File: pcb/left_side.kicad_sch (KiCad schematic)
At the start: 148 parts, among them J1 USB_C_Receptacle_USB2.0_14P, SW1 SW_Push, SW10 SW_Push, SW11 SW_Push, SW12 SW_Push, SW13 SW_Push, SW14 SW_Push, SW15 SW_Push, SW16 SW_Push, SW17 SW_Push, SW18 SW_Push, SW19 SW_Push, SW2 SW_Push, SW20 SW_Push, SW21 SW_Push, SW22 SW_Push, SW23 SW_Push, SW24 SW_Push, SW25 SW_Push, SW26 SW_Push, SW27 SW_Push, SW28 SW_Push, SW29 SW_Push, SW3 SW_Push, SW30 SW_Push, SW31 SW_Push, SW32 SW_Push, SW33 SW_Push, SW34 SW_Push, SW35 SW_Push, SW36 SW_Push, SW37 SW_Push, SW38 SW_Push, SW39 SW_Push, SW4 SW_Push, SW40 SW_Push, SW41 SW_Push, SW42 SW_Push, SW43 SW_Push, SW44 SW_Push, SW45 SW_Push, SW46 SW_Push, SW47 SW_Push, SW48 SW_Push, SW5 SW_Push, SW6 SW_Push, SW7 SW_Push, SW8 SW_Push, SW9 SW_Push

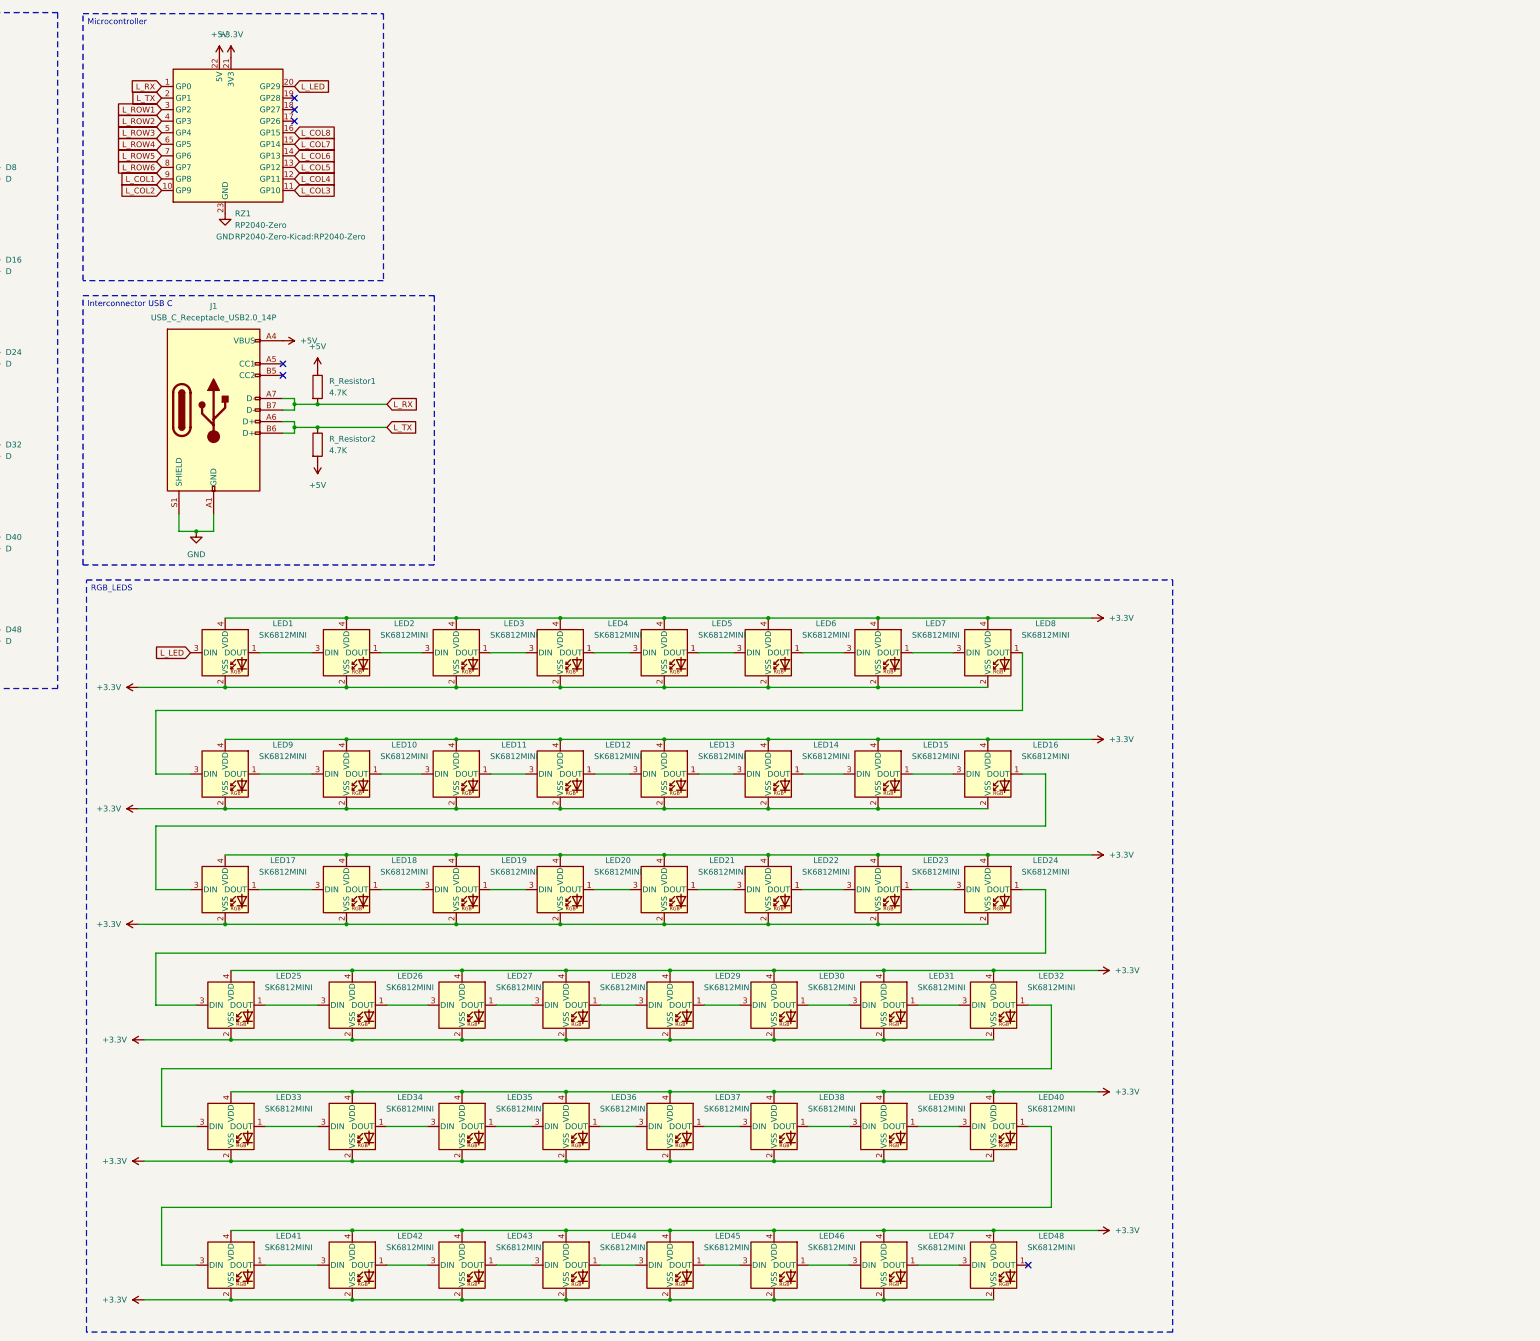
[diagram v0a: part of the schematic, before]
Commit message: update
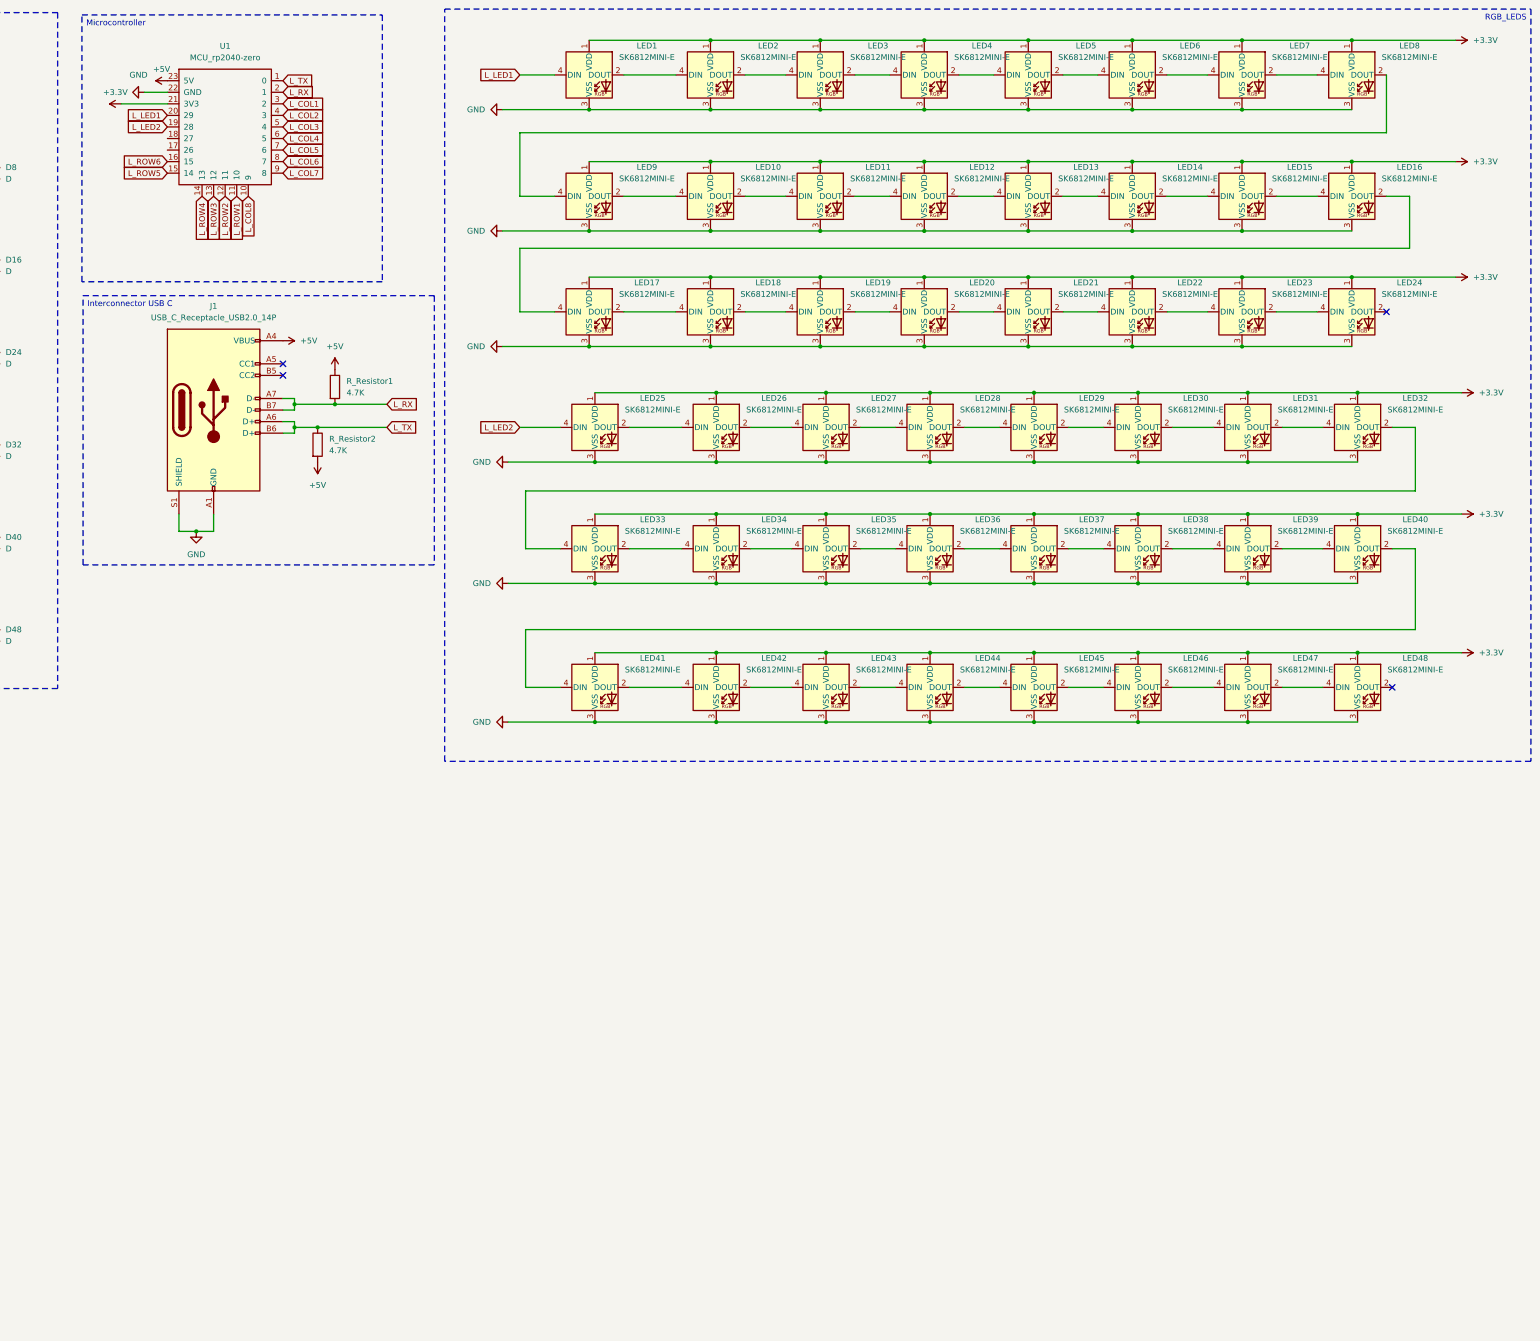
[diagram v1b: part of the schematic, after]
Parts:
- removed LED1, LED10, LED11, LED12, LED13, LED14, LED15, LED16, LED17, LED18, LED19, LED2, LED20, LED21, LED22, LED23, LED24, LED25, LED26, LED27, LED28, LED29, LED3, LED30, LED31, LED32, LED33, LED34, LED35, LED36, LED37, LED38, LED39, LED4, LED40, LED41, LED42, LED43, LED44, LED45, LED46, LED47, LED48, LED5, LED6, LED7, LED8, LED9: SK6812MINI, LED_SMD:LED_SK6812MINI_PLCC4_3.5x3.5mm_P1.75mm, symbol LED:SK6812MINI
- removed RZ1: RP2040-Zero, RP2040-Zero-Kicad:RP2040-Zero, symbol rp2040-zero:RP2040-Zero
- added LED1, LED10, LED11, LED12, LED13, LED14, LED15, LED16, LED17, LED18, LED19, LED2, LED20, LED21, LED22, LED23, LED24, LED25, LED26, LED27, LED28, LED29, LED3, LED30, LED31, LED32, LED33, LED34, LED35, LED36, LED37, LED38, LED39, LED4, LED40, LED41, LED42, LED43, LED44, LED45, LED46, LED47, LED48, LED5, LED6, LED7, LED8, LED9: SK6812MINI-E, SK6812MINI-E:SK6812_mini_e_flipable, symbol SK6812MINI-E:SK6812MINI-E
- added U1: MCU_rp2040-zero, symbol RP2040-Zero:MCU_rp2040-zero
- SW17, SW41, SW42, SW46: footprint MX_Hotswap:MX-Hotswap-1U -> MX_Hotswap:MX-Hotswap-1.25U
- SW25, SW47: footprint MX_Hotswap:MX-Hotswap-1U -> MX_Hotswap:MX-Hotswap-1.5U
- SW33, SW48: footprint MX_Hotswap:MX-Hotswap-1U -> MX_Hotswap:MX-Hotswap-1.75U
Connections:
- net +3.3V: now also LED1.1 (VDD), LED10.1 (VDD), LED11.1 (VDD), LED12.1 (VDD), LED13.1 (VDD), LED14.1 (VDD), LED15.1 (VDD), LED16.1 (VDD), LED17.1 (VDD), LED18.1 (VDD), LED19.1 (VDD), LED2.1 (VDD), LED20.1 (VDD), LED21.1 (VDD), LED22.1 (VDD), LED23.1 (VDD), LED24.1 (VDD), LED25.1 (VDD), LED26.1 (VDD), LED27.1 (VDD), LED28.1 (VDD), LED29.1 (VDD), LED3.1 (VDD), LED30.1 (VDD), LED31.1 (VDD), LED32.1 (VDD), LED33.1 (VDD), LED34.1 (VDD), LED35.1 (VDD), LED36.1 (VDD), LED37.1 (VDD), LED38.1 (VDD), LED39.1 (VDD), LED4.1 (VDD), LED40.1 (VDD), LED41.1 (VDD), LED42.1 (VDD), LED43.1 (VDD), LED44.1 (VDD), LED45.1 (VDD), LED46.1 (VDD), LED47.1 (VDD), LED48.1 (VDD), LED5.1 (VDD), LED6.1 (VDD), LED7.1 (VDD), LED8.1 (VDD), LED9.1 (VDD), U1.21 (3V3)
- net +5V: now also U1.23 (5V)
- net GND: now also LED1.3 (VSS), LED10.3 (VSS), LED11.3 (VSS), LED12.3 (VSS), LED13.3 (VSS), LED14.3 (VSS), LED15.3 (VSS), LED16.3 (VSS), LED17.3 (VSS), LED18.3 (VSS), LED19.3 (VSS), LED2.3 (VSS), LED20.3 (VSS), LED21.3 (VSS), LED22.3 (VSS), LED23.3 (VSS), LED24.3 (VSS), LED25.3 (VSS), LED26.3 (VSS), LED27.3 (VSS), LED28.3 (VSS), LED29.3 (VSS), LED3.3 (VSS), LED30.3 (VSS), LED31.3 (VSS), LED32.3 (VSS), LED33.3 (VSS), LED34.3 (VSS), LED35.3 (VSS), LED36.3 (VSS), LED37.3 (VSS), LED38.3 (VSS), LED39.3 (VSS), LED4.3 (VSS), LED40.3 (VSS), LED41.3 (VSS), LED42.3 (VSS), LED43.3 (VSS), LED44.3 (VSS), LED45.3 (VSS), LED46.3 (VSS), LED47.3 (VSS), LED48.3 (VSS), LED5.3 (VSS), LED6.3 (VSS), LED7.3 (VSS), LED8.3 (VSS), LED9.3 (VSS), U1.22 (GND)
- net L_COL1: now also U1.3 (2)
- net L_COL2: now also U1.4 (3)
- net L_COL3: now also U1.5 (4)
- net L_COL4: now also U1.6 (5)
- net L_COL5: now also U1.7 (6)
- net L_COL6: now also U1.8 (7)
- net L_COL7: now also U1.9 (8)
- net L_COL8: now also U1.10 (9)
- net L_ROW1: now also U1.11 (10)
- net L_ROW2: now also U1.12 (11)
- net L_ROW3: now also U1.13 (12)
- net L_ROW4: now also U1.14 (13)
- net L_ROW5: now also U1.15 (14)
- net L_ROW6: now also U1.16 (15)
- net L_RX: now also U1.2 (1)
- net L_TX: now also U1.1 (0)
- new net: LED31.2 (DOUT), LED32.4 (DIN)
- new net: LED30.2 (DOUT), LED31.4 (DIN)
- new net: LED7.2 (DOUT), LED8.4 (DIN)
- new net: LED6.2 (DOUT), LED7.4 (DIN)
- new net: LED43.2 (DOUT), LED44.4 (DIN)
- new net: LED42.2 (DOUT), LED43.4 (DIN)
- new net: LED19.2 (DOUT), LED20.4 (DIN)
- new net: LED18.2 (DOUT), LED19.4 (DIN)
- new net: LED16.2 (DOUT), LED17.4 (DIN)
- new net: LED15.2 (DOUT), LED16.4 (DIN)
- new net: LED23.2 (DOUT), LED24.4 (DIN)
- new net: LED22.2 (DOUT), LED23.4 (DIN)
- new net: LED11.2 (DOUT), LED12.4 (DIN)
- new net: LED10.2 (DOUT), LED11.4 (DIN)
- new net: LED17.2 (DOUT), LED18.4 (DIN)
- new net: LED10.4 (DIN), LED9.2 (DOUT)
- new net: LED8.2 (DOUT), LED9.4 (DIN)
- new net: LED33.2 (DOUT), LED34.4 (DIN)
- new net: LED32.2 (DOUT), LED33.4 (DIN)
- new net: LED21.2 (DOUT), LED22.4 (DIN)
- new net: LED4.2 (DOUT), LED5.4 (DIN)
- new net: LED3.2 (DOUT), LED4.4 (DIN)
- new net: LED36.2 (DOUT), LED37.4 (DIN)
- new net: LED35.2 (DOUT), LED36.4 (DIN)
- new net: LED47.2 (DOUT), LED48.4 (DIN)
- new net: LED37.2 (DOUT), LED38.4 (DIN)
- new net: LED20.2 (DOUT), LED21.4 (DIN)
- new net: LED27.2 (DOUT), LED28.4 (DIN)
- new net: LED26.2 (DOUT), LED27.4 (DIN)
- new net: LED46.2 (DOUT), LED47.4 (DIN)
- new net: LED34.2 (DOUT), LED35.4 (DIN)
- new net: LED14.2 (DOUT), LED15.4 (DIN)
- new net: LED13.2 (DOUT), LED14.4 (DIN)
- new net: LED41.2 (DOUT), LED42.4 (DIN)
- new net: LED40.2 (DOUT), LED41.4 (DIN)
- new net: LED12.2 (DOUT), LED13.4 (DIN)
- new net: LED38.2 (DOUT), LED39.4 (DIN)
- new net: LED5.2 (DOUT), LED6.4 (DIN)
- new net: LED45.2 (DOUT), LED46.4 (DIN)
- new net: LED44.2 (DOUT), LED45.4 (DIN)
- new net: LED29.2 (DOUT), LED30.4 (DIN)
- new net: LED25.2 (DOUT), LED26.4 (DIN)
- new net: LED39.2 (DOUT), LED40.4 (DIN)
- new net: LED28.2 (DOUT), LED29.4 (DIN)
- new net: LED2.2 (DOUT), LED3.4 (DIN)
- new net: LED1.2 (DOUT), LED2.4 (DIN)
- new net L_LED1: LED1.4 (DIN), U1.20 (29)
- new net L_LED2: LED25.4 (DIN), U1.19 (28)
- no-connect marks 6 -> 4
